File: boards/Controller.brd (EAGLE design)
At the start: 101.6 x 152.4 mm, 119 parts, among them J1 RJ45-8PTH, J10 MOLEX-70545-02POSITION, J11 MOLEX-70545-02POSITION, J12 MOLEX-70545-02POSITION, J15 MOLEX-70545-02POSITION, J16 MOLEX-70545-02POSITION, J17 MOLEX-70545-02POSITION, J18 MOLEX-70545-02POSITION, J19 MOLEX-70545-02POSITION, J2 RJ45-8PTH, J20 MOLEX-70545-02POSITION, J3 MOLEX-70545-02POSITION, J4 MOLEX-70545-02POSITION, J5 MOLEX-70545-02POSITION, J6 MOLEX-70545-02POSITION, J7 MOLEX-70545-02POSITION, J8 MOLEX-70545-02POSITION, J9 MOLEX-70545-02POSITION, Q2 MPSA27, U2 7805, U3 SN75176BP, U4 ATMEGA128-SMD, X3 5566-8, X4 5566-8, Y1 16MHz

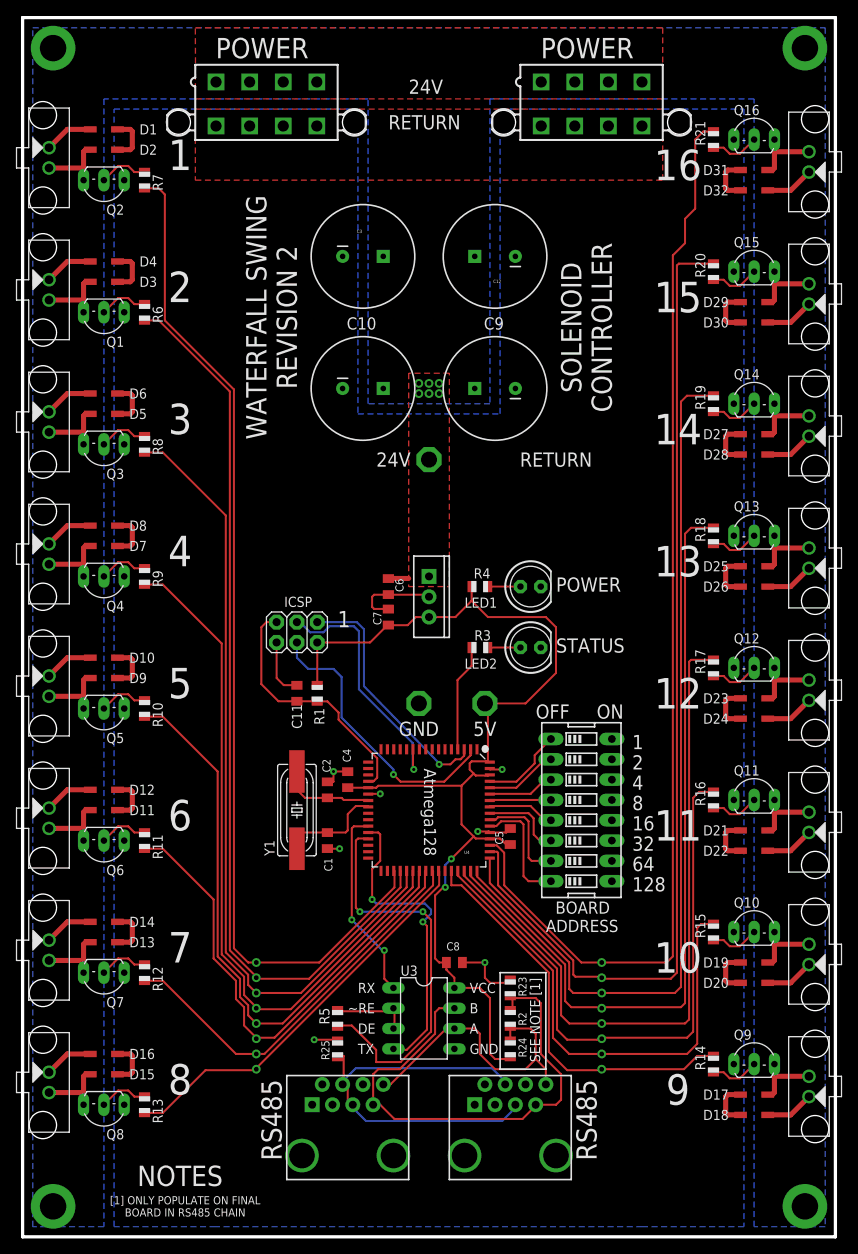
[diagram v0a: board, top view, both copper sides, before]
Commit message: put all the downloaded files into directories
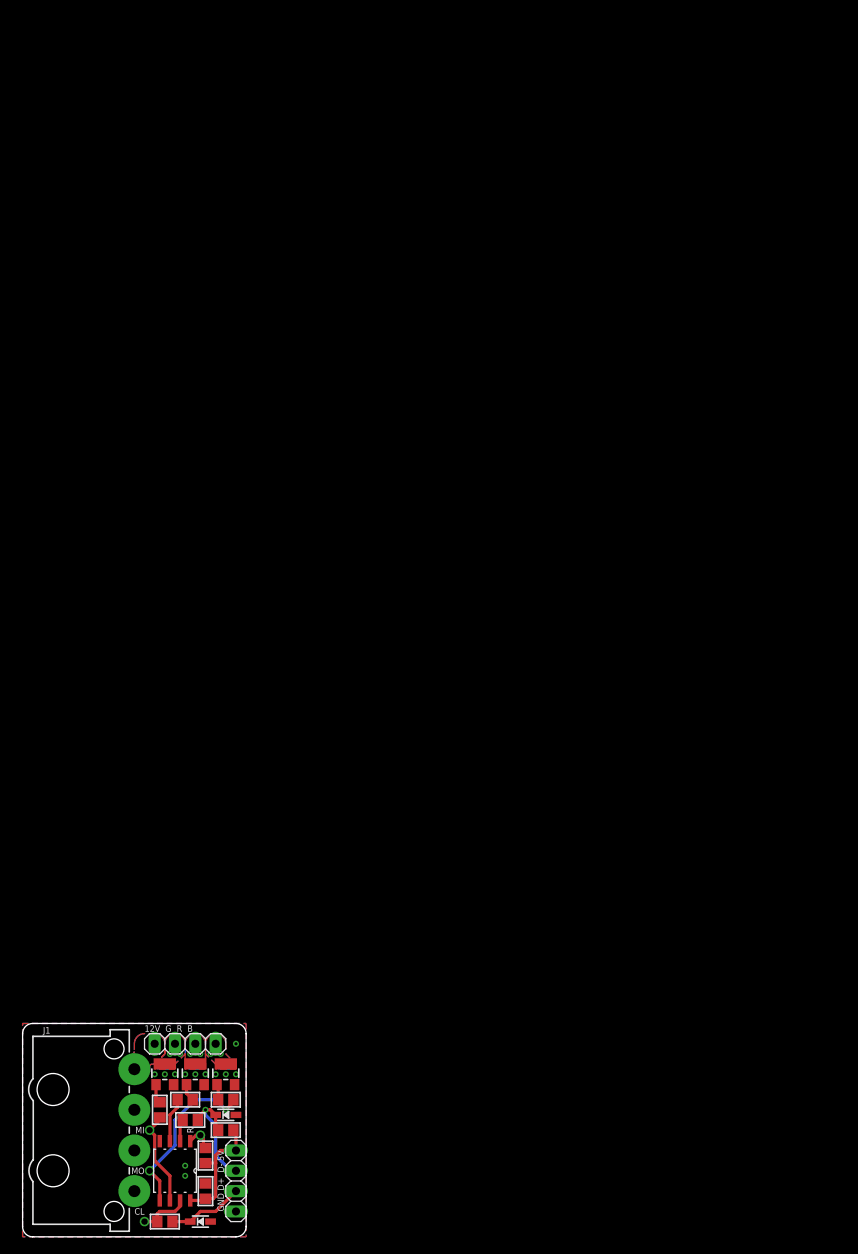
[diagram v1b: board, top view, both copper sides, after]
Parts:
- removed C10, C12, C3, C9: 1000u, custom:CPOL-RADIAL-1000UF-35V
- removed C11, C4, C5, C8: .1u, adafruit:C0805K
- removed C2: 33p, adafruit:C0805K
- removed C6, C7: 15uF, 25V, adafruit:C0805K
- removed D10, D11, D12, D13, D14, D15, D16, D17, D18, D19, D20, D21, D22, D23, D24, D25, D26, D27, D28, D29, D3, D30, D31, D32, D4, D5, D6, D7, D8, D9: (no value), semicon-smd-ipc:SOD123
- removed ICSP: (no value), SparkFun:2X03
- removed J10, J11, J12, J15, J16, J17, J18, J19, J20, J3, J4, J5, J6, J7, J8, J9: MOLEX-70545-02POSITION, icc:MOLEX-70545-02POSITION
- removed J2: RJ45-8PTH, custom:RJ45-8
- removed JP3, JP4: STAND-OFF, custom:STAND-OFF
- removed LED1, LED2: (no value), adafruit:LED5MM
- removed Q10, Q11, Q12, Q13, Q14, Q15, Q16, Q4, Q5, Q6, Q7, Q8, Q9: (no value), transistor-neu-to92:TO92-EBC
- removed R10, R11, R12, R13, R14, R15, R16, R17, R18, R19, R20, R21, R8, R9: 10k, adafruit:R0805
- removed R23, R24: 560, adafruit:R0805
- removed R25: 0, adafruit:R0805
- removed SW1: (no value), SparkFun-Electromechanical:DIPSWITCH-08
- removed TP1, TP3, TP4: PTR1PAD1-20, testpad:P1-20
- removed U2: 7805, SparkFun:TO220-IGO
- removed U3: SN75176BP, custom:DIL08
- removed U4: ATMEGA128-SMD, SparkFun-DigitalIC:TQFP64_14X14MM
- removed X3, X4: 5566-8, con-molex:5566-8
- removed Y1: 16MHz, crystal:HC49UP
- added U1: ATTINY85, zak:SOIC127P798X216-8N
- C1: value 33p -> 1u; device adafruit:C0805K -> microbuilder:0805
- D1, D2: value (none) -> 3V6; device semicon-smd-ipc:SOD123 -> zak:SOD-323
- J1: value RJ45-8PTH -> PWR; device custom:RJ45-8 -> con-amp:827001
- JP1: value STAND-OFF -> USB; device custom:STAND-OFF -> pinhead:1X04
- JP2: value STAND-OFF -> LED; device custom:STAND-OFF -> pinhead:1X04
- Q1, Q3: value (none) -> DMG6968U; device transistor-neu-to92:TO92-EBC -> microbuilder:SOT23-W
- Q2: value MPSA27 -> DMG6968U; device transistor-neu-to92:TO92-EBC -> microbuilder:SOT23-W
- R1: value 10k -> 150R; device adafruit:R0805 -> microbuilder:0805
- R2: value 120 -> 150R; device adafruit:R0805 -> microbuilder:0805
- R3: value 1k -> 150R; device adafruit:R0805 -> microbuilder:0805
- R4, R5: value 1k -> 100R; device adafruit:R0805 -> microbuilder:0805
- R6: value 10k -> 2K2; device adafruit:R0805 -> microbuilder:0805
- R7: value 10k -> 10K; device adafruit:R0805 -> microbuilder:0805
- moved D2 134.5 mm to (22.2, 1.91)
- moved D1 124.1 mm to (25.4, 15.2)
- moved R7 122.2 mm to (22.9, 10.2)
- moved Q2 111.1 mm to (21.6, 20.3), turned to 0 degrees
- moved R6 102.7 mm to (25.4, 13.3), turned to 0 degrees
- moved Q1 94.3 mm to (17.8, 20.3), turned to 0 degrees
- moved Q3 79.0 mm to (25.4, 20.3), turned to 0 degrees
- moved R4 75.9 mm to (21.0, 14.6)
- moved JP1 71.2 mm to (26.7, 6.99), turned to 270 degrees
- moved R3 64.8 mm to (25.4, 17.1)
- moved R1 55.7 mm to (17.1, 15.9), turned to 90 degrees
- moved C1 46.4 mm to (22.9, 5.71), turned to 90 degrees
- moved R2 41.9 mm to (20.3, 17.1), turned to 0 degrees
- moved R5 33.3 mm to (17.8, 1.91), turned to 0 degrees
- moved J1 26.9 mm to (14.0, 13.3), turned to 270 degrees
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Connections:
- removed net 5V: C4.1, C5.1, C7.1, C8.1, ICSP.2, R1.1, R24.2, R4.1, TP3.TP, U2.OUT, U3.8, U4.21, U4.52, U4.62, U4.64
- removed net A: J1.8, J2.8, R2.2, R24.1, U3.6
- removed net B: J1.7, J2.7, R2.1, R23.2, U3.7
- removed net N$11: Q2.B, R7.1
- removed net N$12: R5.2, U3.2, U3.3
- removed net N$13: D3.1, J4.P2, Q1.C
- removed net N$14: D2.1, J3.P2, Q2.C
- removed net N$16: D10.2, D9.2
- removed net N$17: D1.2, D2.2
- removed net N$18: Q3.B, R8.1
- removed net N$19: D5.1, J5.P2, Q3.C
- removed net N$20: D17.2, D18.2
- removed net N$21: Q4.B, R9.1
- removed net N$22: D7.1, J6.P2, Q4.C
- removed net N$23: D25.2, D26.2
- removed net N$24: Q5.B, R10.1
- removed net N$25: D9.1, J7.P2, Q5.C
- removed net N$26: D27.2, D28.2
- removed net N$27: Q6.B, R11.1
- removed net N$28: D11.1, J8.P2, Q6.C
- removed net N$29: D19.2, D20.2
- removed net N$30: Q7.B, R12.1
- removed net N$31: D13.1, J9.P2, Q7.C
- removed net N$32: D11.2, D12.2
- removed net N$33: Q8.B, R13.1
- removed net N$34: D15.1, J10.P2, Q8.C
- removed net N$35: D3.2, D4.2
- removed net N$36: Q9.B, R14.1
- removed net N$37: D17.1, J11.P2, Q9.C
- removed net N$38: D5.2, D6.2
- removed net N$39: Q10.B, R15.1
- removed net N$4: U3.4, U4.28
- removed net N$40: D19.1, J12.P2, Q10.C
- removed net N$41: D13.2, D14.2
- removed net N$42: Q11.B, R16.1
- removed net N$43: D21.1, J15.P2, Q11.C
- removed net N$44: D21.2, D22.2
- removed net N$45: Q12.B, R17.1
- removed net N$46: D23.1, J16.P2, Q12.C
- removed net N$47: D29.2, D30.2
- removed net N$48: Q13.B, R18.1
- removed net N$49: D25.1, J17.P2, Q13.C
- removed net N$5: C2.1, U4.23, Y1.2
- removed net N$50: D31.2, D32.2
- removed net N$51: Q14.B, R19.1
- removed net N$52: D27.1, J18.P2, Q14.C
- removed net N$53: D23.2, D24.2
- removed net N$54: Q15.B, R20.1
- removed net N$55: D29.1, J19.P2, Q15.C
- removed net N$56: D15.2, D16.2
- removed net N$57: Q16.B, R21.1
- removed net N$58: D31.1, J20.P2, Q16.C
- removed net N$59: D7.2, D8.2
- removed net N$6: C1.1, U4.24, Y1.1
- removed net N$60: J1.4, J1.5, J2.4, J2.5, R25.1
- removed net N$61: SW1.1, U4.61
- removed net N$62: SW1.2, U4.60
- removed net N$63: SW1.3, U4.59
- removed net N$64: SW1.4, U4.58
- removed net N$65: SW1.5, U4.57
- removed net N$66: SW1.6, U4.56
- removed net N$67: SW1.7, U4.55
- removed net N$68: SW1.8, U4.54
- removed net N$70: R5.1, U4.29
- removed net NRESET: C11.1, ICSP.5, R1.2, U4.20
- removed net V+: C10.1, C12.1, C3.1, C6.1, C9.1, D1.1, D10.1, D12.1, D14.1, D16.1, D18.1, D20.1, D22.1, D24.1, D26.1, D28.1, D30.1, D32.1, D4.1, D6.1, D8.1, J10.P1, J11.P1, J12.P1, J15.P1, J16.P1, J17.P1, J18.P1, J19.P1, J20.P1, J3.P1, J4.P1, J5.P1, J6.P1, J7.P1, J8.P1, J9.P1, TP1.TP, U2.IN, X3.1, X3.2, X3.3, X3.4, X4.1, X4.2, X4.3, X4.4
- removed net VALVE1: R7.2, U4.35
- removed net VALVE10: R15.2, U4.45
- removed net VALVE11: R16.2, U4.46
- removed net VALVE12: R17.2, U4.47
- removed net VALVE13: R18.2, U4.48
- removed net VALVE14: R19.2, U4.49
- removed net VALVE15: R20.2, U4.50
- removed net VALVE16: R21.2, U4.51
- removed net VALVE2: R6.2, U4.36
- removed net VALVE3: R8.2, U4.37
- removed net VALVE4: R9.2, U4.38
- removed net VALVE5: R10.2, U4.39
- removed net VALVE6: R11.2, U4.40
- removed net VALVE7: R12.2, U4.41
- removed net VALVE8: R13.2, U4.42
- removed net VALVE9: R14.2, U4.44
- new net +5V: C1.1, JP1.1, R6.2, R7.2, U1.8
- new net BLUE: JP2.4, Q3.3
- new net D+: D2.C, JP1.3, R5.2
- new net D-: D1.C, JP1.2, R4.2, R6.1
- new net GREEN: JP2.2, Q1.3
- new net N$2: Q2.1, R2.2
- new net RED: JP2.3, Q2.3
- new net RST: R7.1, U1.1
- net GND: now also D1.A, D2.A, J1.2, JP1.4, Q1.2, Q2.2, Q3.2, U1.4; no longer C10.2, C11.2, C12.2, C2.2, C3.2, C4.2, C5.2, C6.2, C7.2, C8.2, C9.2, ICSP.6, LED1.K, LED2.K, Q1.E, Q10.E, Q11.E, Q12.E, Q13.E, Q14.E, Q15.E, Q16.E, Q2.E, Q3.E, Q4.E, Q5.E, Q6.E, Q7.E, Q8.E, Q9.E, R23.1, R25.2, SW1.10, SW1.11, SW1.12, SW1.13, SW1.14, SW1.15, SW1.16, SW1.9, TP4.TP, U2.GND, U3.5, U4.22, U4.53, U4.63, X3.5, X3.6, X3.7, X3.8, X4.5, X4.6, X4.7, X4.8
- net MISO: now also R1.1, U1.6; no longer ICSP.1, U4.3
- net MOSI: now also R3.1, U1.5; no longer ICSP.4, U4.2
- net N$1: now also Q1.1, R1.2; no longer U3.1, U4.27
- net N$3: now also Q3.1; no longer U4.4
- net N$7: now also R4.1, U1.2; no longer LED1.A, R4.2
- net N$8: now also J1.1, JP2.1; no longer LED2.A, R3.1
- net N$9: now also R2.1, U1.3; no longer Q1.B, R6.1
- net SCK: now also R5.1, U1.7; no longer ICSP.3, U4.11
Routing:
- net VALVE16: track 137.6 -> 0.00 mm, vias 1 -> 0
- net 5V: track 137.0 -> 0.00 mm, vias 2 -> 0
- net VALVE1: track 127.5 -> 0.00 mm, vias 1 -> 0
- net VALVE15: track 126.8 -> 0.00 mm, vias 1 -> 0
- net VALVE2: track 114.0 -> 0.00 mm, vias 1 -> 0
- net VALVE14: track 112.5 -> 0.00 mm, vias 1 -> 0
- net VALVE3: track 101.0 -> 0.00 mm, vias 1 -> 0
- net V+: track 100.2 -> 0.00 mm, vias 6 -> 0
- net VALVE13: track 99.1 -> 0.00 mm, vias 1 -> 0
- net VALVE4: track 88.2 -> 0.00 mm, vias 1 -> 0
- net VALVE12: track 87.2 -> 0.00 mm, vias 1 -> 0
- net VALVE11: track 75.2 -> 0.00 mm, vias 1 -> 0
- net VALVE5: track 75.0 -> 0.00 mm, vias 1 -> 0
- net B: track 63.5 -> 0.00 mm
- net VALVE6: track 61.9 -> 0.00 mm, vias 1 -> 0
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- added copper zone on layer 1, net BLUE
- added copper zone on layer 16, net BLUE
- added copper zone on layer 1, net GREEN
- added copper zone on layer 16, net GREEN
- added copper zone on layer 1, net N$8
- added copper zone on layer 16, net N$8
- added copper zone on layer 1, net RED
- added copper zone on layer 16, net RED
- removed copper zone on layer 1, net V+
- removed copper zone on layer 16, net V+
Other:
- board size 101.6 x 152.4 mm -> 27.9 x 26.7 mm
- board text added: "12V G R B"
- board text added: "2013-07-17"
- board text added: "CL"
- board text added: "GND D+ D- 5V"
- board text added: "MI"
- board text added: "MO"
- board text added: "R"
- board text added: "RGB LED Controller"
- board text added: "v1.0"
- board text added: "zakkemble.co.uk"
- board text removed: "1"
- board text removed: "10"
- board text removed: "11"
- board text removed: "12"
- board text removed: "128"
- board text removed: "13"
- board text removed: "14"
- board text removed: "15"
- board text removed: "16"
- board text removed: "2"
- board text removed: "24V"
- board text removed: "3"
- board text removed: "32"
- board text removed: "4"
- board text removed: "5"
- board text removed: "5V"
- board text removed: "6"
- board text removed: "64"
- board text removed: "7"
- board text removed: "8"
- board text removed: "9"
- board text removed: "A"
- board text removed: "Atmega128"
- board text removed: "B"
- board text removed: "BOARD ADDRESS"
- board text removed: "DE"
- board text removed: "GND"
- board text removed: "NOTES"
- board text removed: "OFF"
- board text removed: "ON"
- board text removed: "POWER"
- board text removed: "RETURN"
- board text removed: "RS485"
- board text removed: "RX"
- board text removed: "SEE NOTE [1]"
- board text removed: "SOLENOID CONTROLLER"
- board text removed: "STATUS"
- board text removed: "TX"
- board text removed: "VCC"
- board text removed: "WATERFALL SWING REVISION 2"
- board text removed: "[1] ONLY POPULATE ON FINAL BOARD IN RS485 CHAIN"
- board text removed: "~RE"
- board text removed: "•"
